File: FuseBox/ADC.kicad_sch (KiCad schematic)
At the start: 2 parts, among them U15 OPA1612AIDRGR, U56 PCM1803ADB

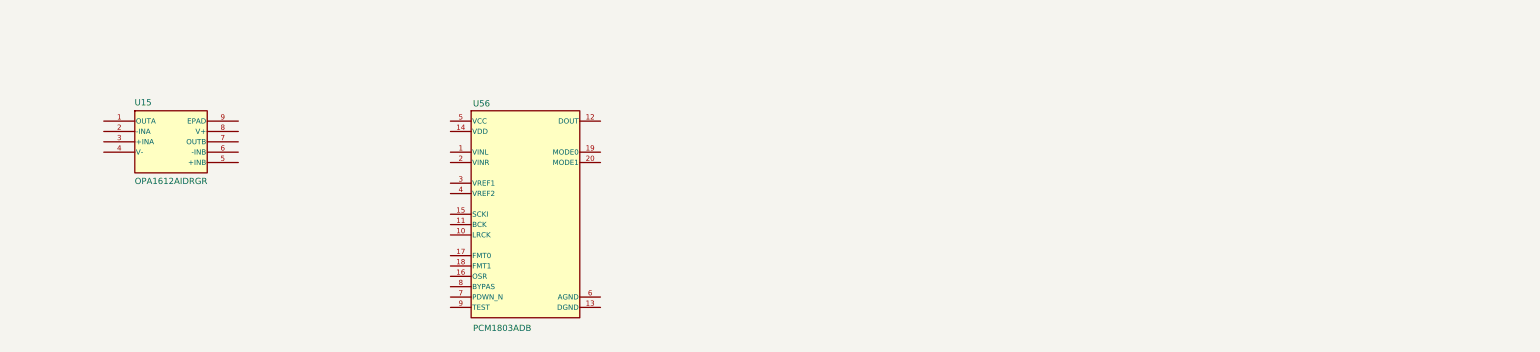
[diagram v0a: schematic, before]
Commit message: stupid analog
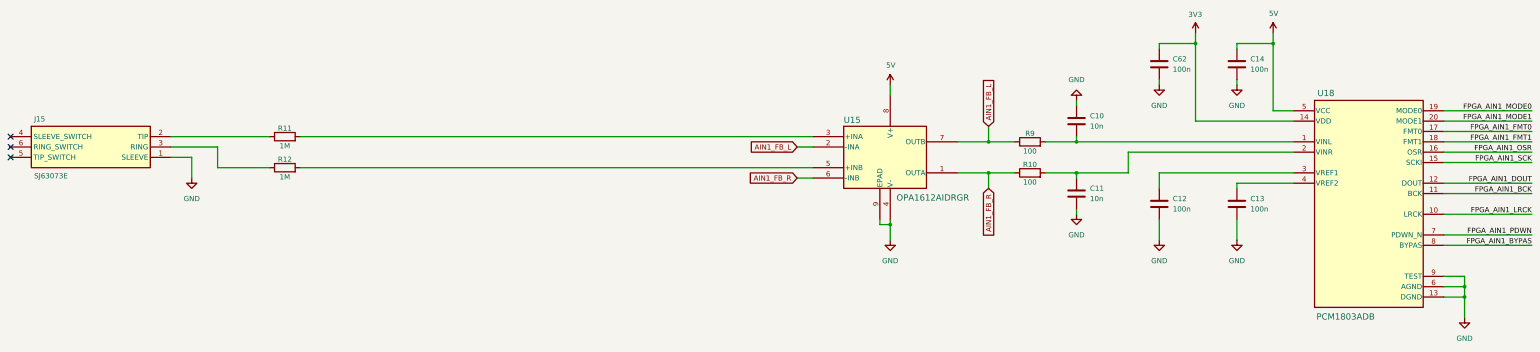
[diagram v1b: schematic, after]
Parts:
- removed U56: PCM1803ADB, Custom:PCM1803ADB, symbol Custom:PCM1803ADB
- added C10, C11: 10n, Capacitor_SMD:C_0603_1608Metric_Pad1.08x0.95mm_HandSolder, symbol Device:C
- added C12, C13, C14, C62: 100n, Capacitor_SMD:C_0603_1608Metric_Pad1.08x0.95mm_HandSolder, symbol Device:C
- added J15: SJ63073E, Custom:SJ63073E, symbol Custom:SJ63073E
- added R10, R9: 100, Resistor_SMD:R_0603_1608Metric_Pad0.98x0.95mm_HandSolder, symbol Device:R
- added R11, R12: 1M, Resistor_SMD:R_0603_1608Metric_Pad0.98x0.95mm_HandSolder, symbol Device:R
- added U18: PCM1803ADB, Custom:PCM1803ADB, symbol Custom:PCM1803ADB
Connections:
- net AIN1_FB_R: now reaches U15.1 (OUTA)
- net AIN1_FB_R: now also U15.6 (-INB), R10.1
- net AIN1_FB_L: now reaches U15.2 (-INA)
- net AIN1_FB_L: now also U15.7 (OUTB), R9.1
- net at U15.3 (+INA): now also R11.2
- net GND: now reaches U15.4 (V-)
- net GND: now also U15.9 (EPAD), C10.1, C11.2, C12.2, C13.2, C14.2, C62.2, J15.1 (SLEEVE), U18.13 (DGND), U18.6 (AGND), U18.9 (TEST)
- net at U15.5 (+INB): now also R12.2
- net 5V: now reaches U15.8 (V+)
- net 5V: now also C14.1, U18.5 (VCC)
- new net: C10.2, R9.2, U18.1 (VINL)
- new net: C11.1, R10.2, U18.2 (VINR)
- new net: C12.1, U18.3 (VREF1)
- new net: C13.1, U18.4 (VREF2)
- new net: J15.3 (RING), R12.1
- new net: J15.2 (TIP), R11.1
- new net 3V3: C62.1, U18.14 (VDD)
- new net FPGA_AIN1_BCK: U18.11 (BCK)
- new net FPGA_AIN1_BYPAS: U18.8 (BYPAS)
- new net FPGA_AIN1_DOUT: U18.12 (DOUT)
- new net FPGA_AIN1_FMT0: U18.17 (FMT0)
- new net FPGA_AIN1_FMT1: U18.18 (FMT1)
- new net FPGA_AIN1_LRCK: U18.10 (LRCK)
- new net FPGA_AIN1_MODE0: U18.19 (MODE0)
- new net FPGA_AIN1_MODE1: U18.20 (MODE1)
- new net FPGA_AIN1_OSR: U18.16 (OSR)
- new net FPGA_AIN1_PDWN: U18.7 (PDWN_N)
- new net FPGA_AIN1_SCK: U18.15 (SCKI)
- no-connect marks 0 -> 3
